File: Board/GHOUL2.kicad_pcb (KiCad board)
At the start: 2 copper layers, 105.4 x 88.9 mm, 21 parts

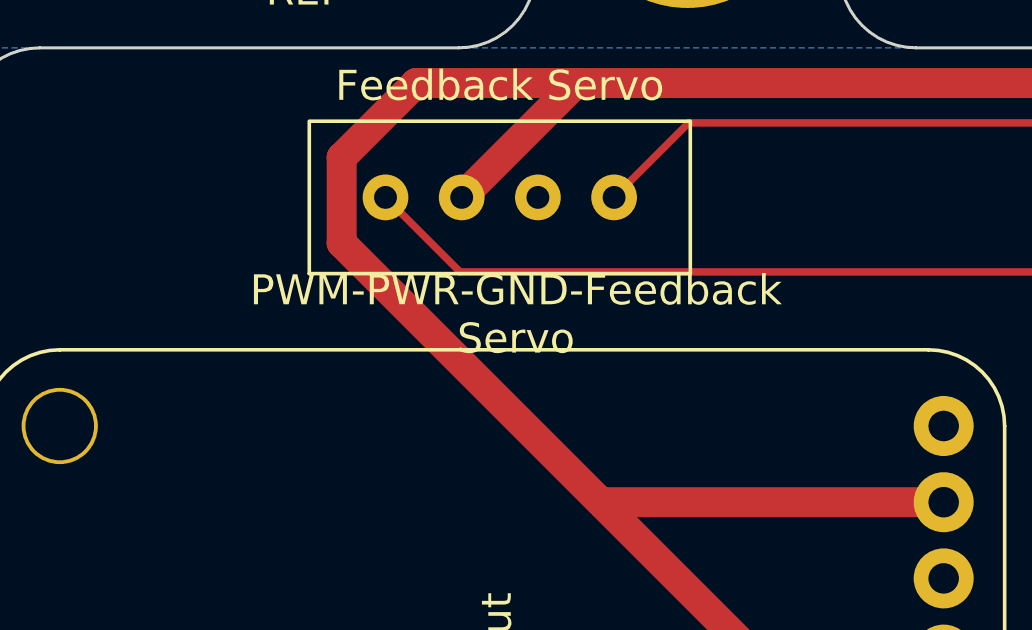
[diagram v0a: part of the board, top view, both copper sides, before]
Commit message: i think we are pretty close to being done
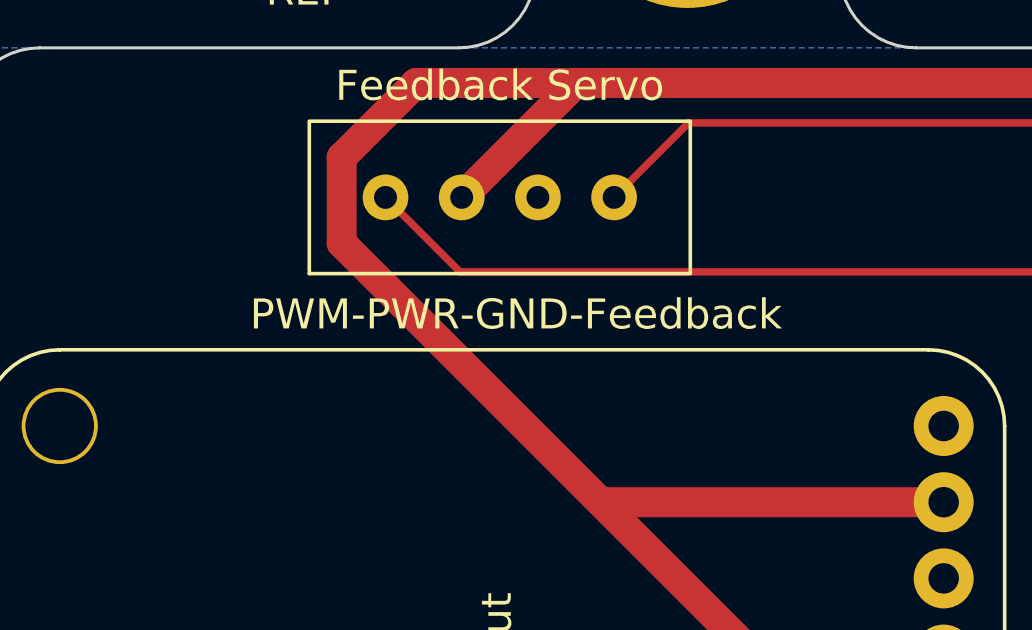
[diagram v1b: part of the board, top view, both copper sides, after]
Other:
- board text added: "PWM-PWR-GND-Feedback"
- board text removed: "PWM-PWR-GND-Feedback Servo"
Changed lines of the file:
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@@
     (effects (font (size 1 1) (thickness 0.15)) (justify left mirror))
   )
-  (gr_text "PWM-PWR-GND-Feedback\nServo" (at 112.395 77.47) (layer "F.SilkS")
+  (gr_text "PWM-PWR-GND-Feedback" (at 112.395 77.47) (layer "F.SilkS")
     (effects (font (size 1 1) (thickness 0.15)))
   )
